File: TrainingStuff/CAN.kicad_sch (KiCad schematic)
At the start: 7 parts, among them U1 OKI

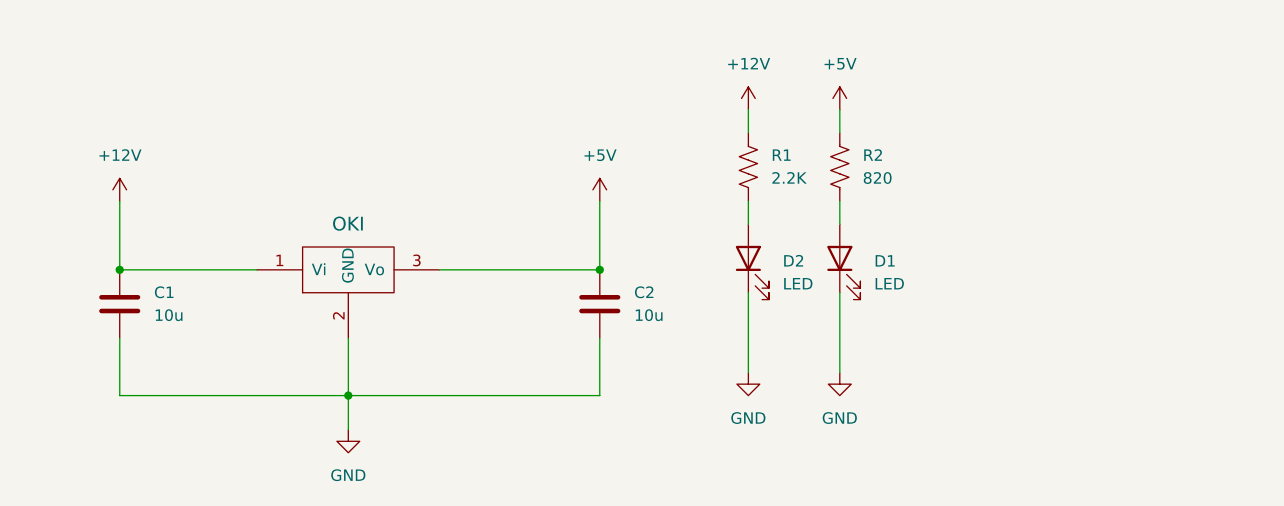
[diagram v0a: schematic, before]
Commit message: Add Schematic
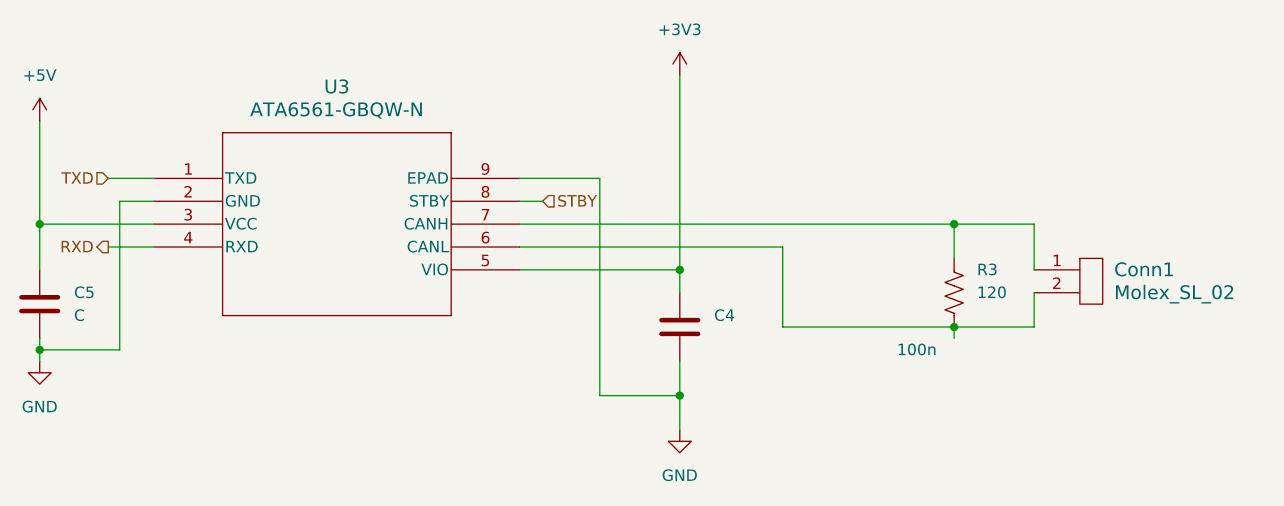
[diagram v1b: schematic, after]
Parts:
- removed C1, C2: 10u, symbol Device:C
- removed D1, D2: LED, symbol Device:LED
- removed R1: 2.2K, symbol Device:R_US
- removed R2: 820, symbol Device:R_US
- removed U1: OKI, symbol MRDT_Devices:OKI
- added C4: 100n, symbol Device:C
- added C5: C, symbol Device:C
- added Conn1: Molex_SL_02, symbol MRDT_Connectors:Molex_SL_02
- added R3: 120, symbol Device:R_US
- added U3: ATA6561-GBQW-N, VDFN8_3X3_MCH, symbol 2026_traning_hardware:ATA6561-GBQW-N
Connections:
- net +5V: now also C5.1, U3.3 (VCC)
- net GND: now also C4.2, C5.2, U3.2 (GND), U3.9 (EPAD)
- new net: Conn1.1, R3.1, U3.7 (CANH)
- new net: Conn1.2, R3.2, U3.6 (CANL)
- new net +3V3: C4.1, U3.5 (VIO)
- new net RXD: U3.4 (RXD)
- new net STBY: U3.8 (STBY)
- new net TXD: U3.1 (TXD)
